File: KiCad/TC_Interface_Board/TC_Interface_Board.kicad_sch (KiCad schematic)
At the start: 23 parts, among them J1_24V_ROW1 Conn_01x04, J1_CN1_24V1 Conn_01x03, J2_CN2_9V_Main1 Conn_01x02, J3_CN3_9V_Main1 Conn_01x02, J4_BUS_MONITER1 Conn_01x05, Q1 DTC143E, Q2 DTC143E, U1 MC34063AP

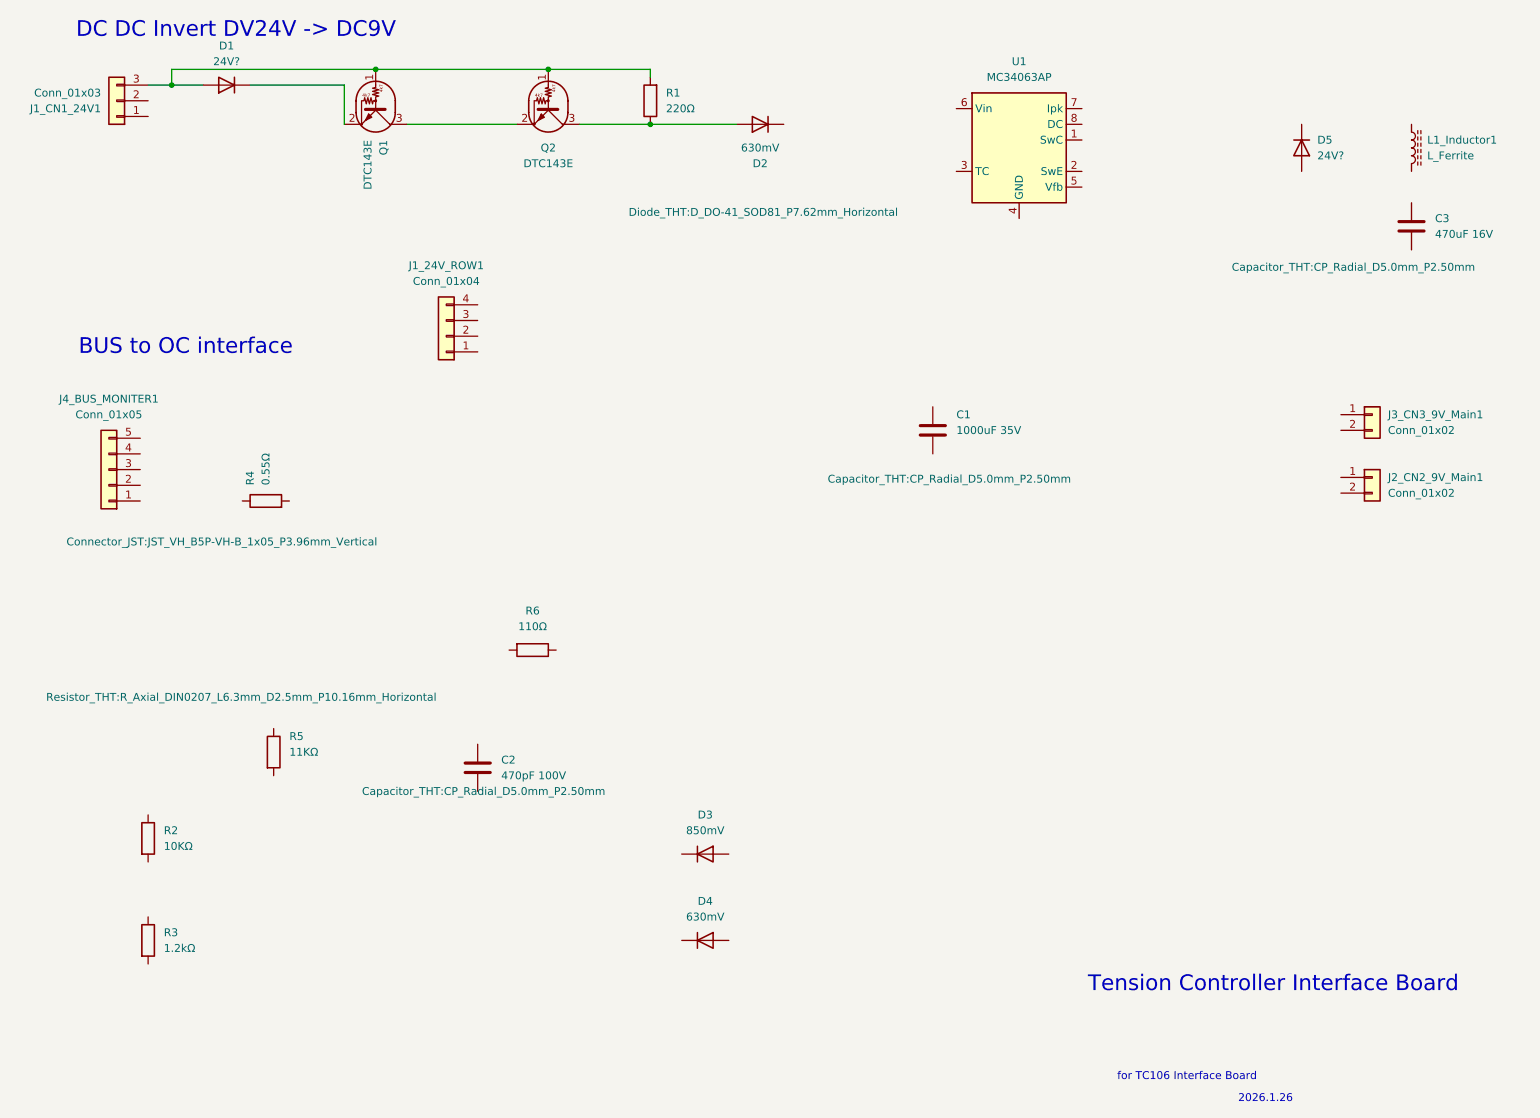
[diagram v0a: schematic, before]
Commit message: UPDATE
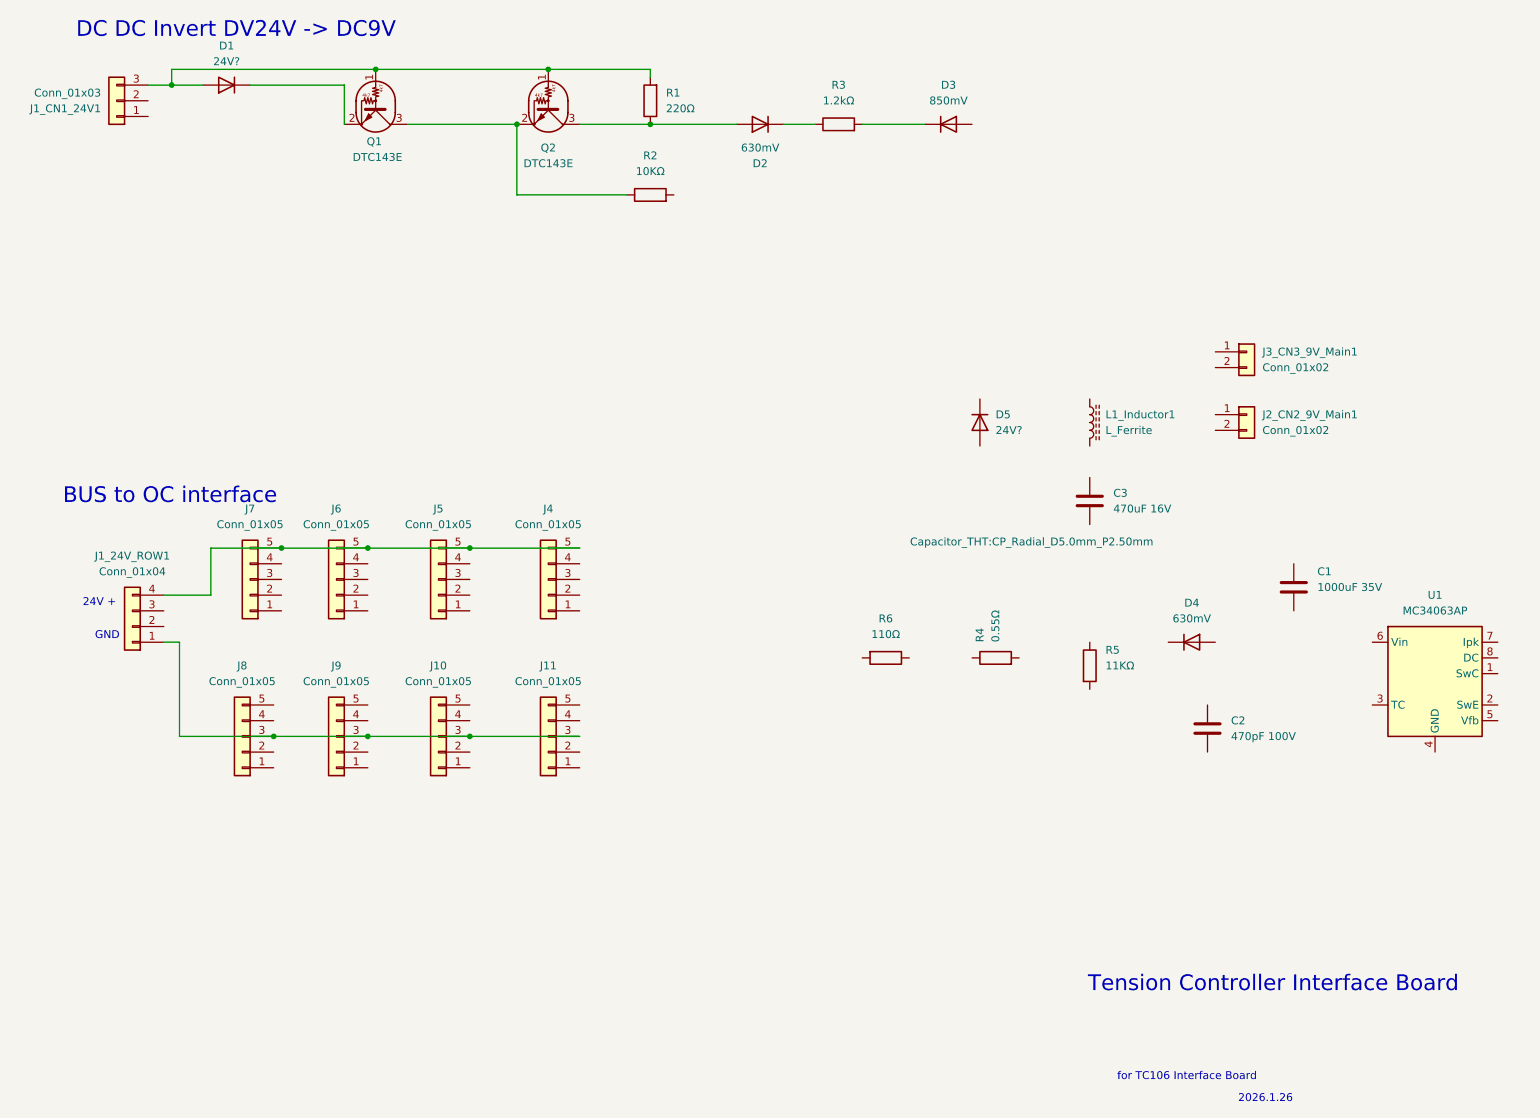
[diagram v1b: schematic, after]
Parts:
- added J10, J11, J5, J6, J7, J8, J9: Conn_01x05, Connector_JST:JST_VH_B5P-VH-B_1x05_P3.96mm_Vertical, symbol Connector_Generic:Conn_01x05
- D3: footprint Diode_THT:D_DO-41_SOD81_P7.62mm_Horizontal -> Diode_THT:D_DO-41_SOD81_P10.16mm_Horizontal
- R3: footprint Resistor_THT:R_Axial_DIN0207_L6.3mm_D2.5mm_P7.62mm_Horizontal -> Resistor_THT:R_Axial_DIN0207_L6.3mm_D2.5mm_P15.24mm_Horizontal
- renumbered J4_BUS_MONITER1 to J4
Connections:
- net at R3.1: now also D2.1 (K)
- net at R3.2: now also D3.1 (K)
- net at Q1.3 (C), Q2.2 (E): now also R2.1
- net at J1_24V_ROW1.1 (Pin_1): now also J10.3 (Pin_3), J11.3 (Pin_3), J8.3 (Pin_3), J9.3 (Pin_3)
- net at J1_24V_ROW1.4 (Pin_4): now also J4.5 (Pin_5), J5.5 (Pin_5), J6.5 (Pin_5), J7.5 (Pin_5)
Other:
- note added: "24V +"
- note added: "GND"
- moved on the sheet: C1, C2, C3, D3, D4, D5, J1_24V_ROW1, J2_CN2_9V_Main1, J3_CN3_9V_Main1, J4, L1_Inductor1, R2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

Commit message: UPDATE
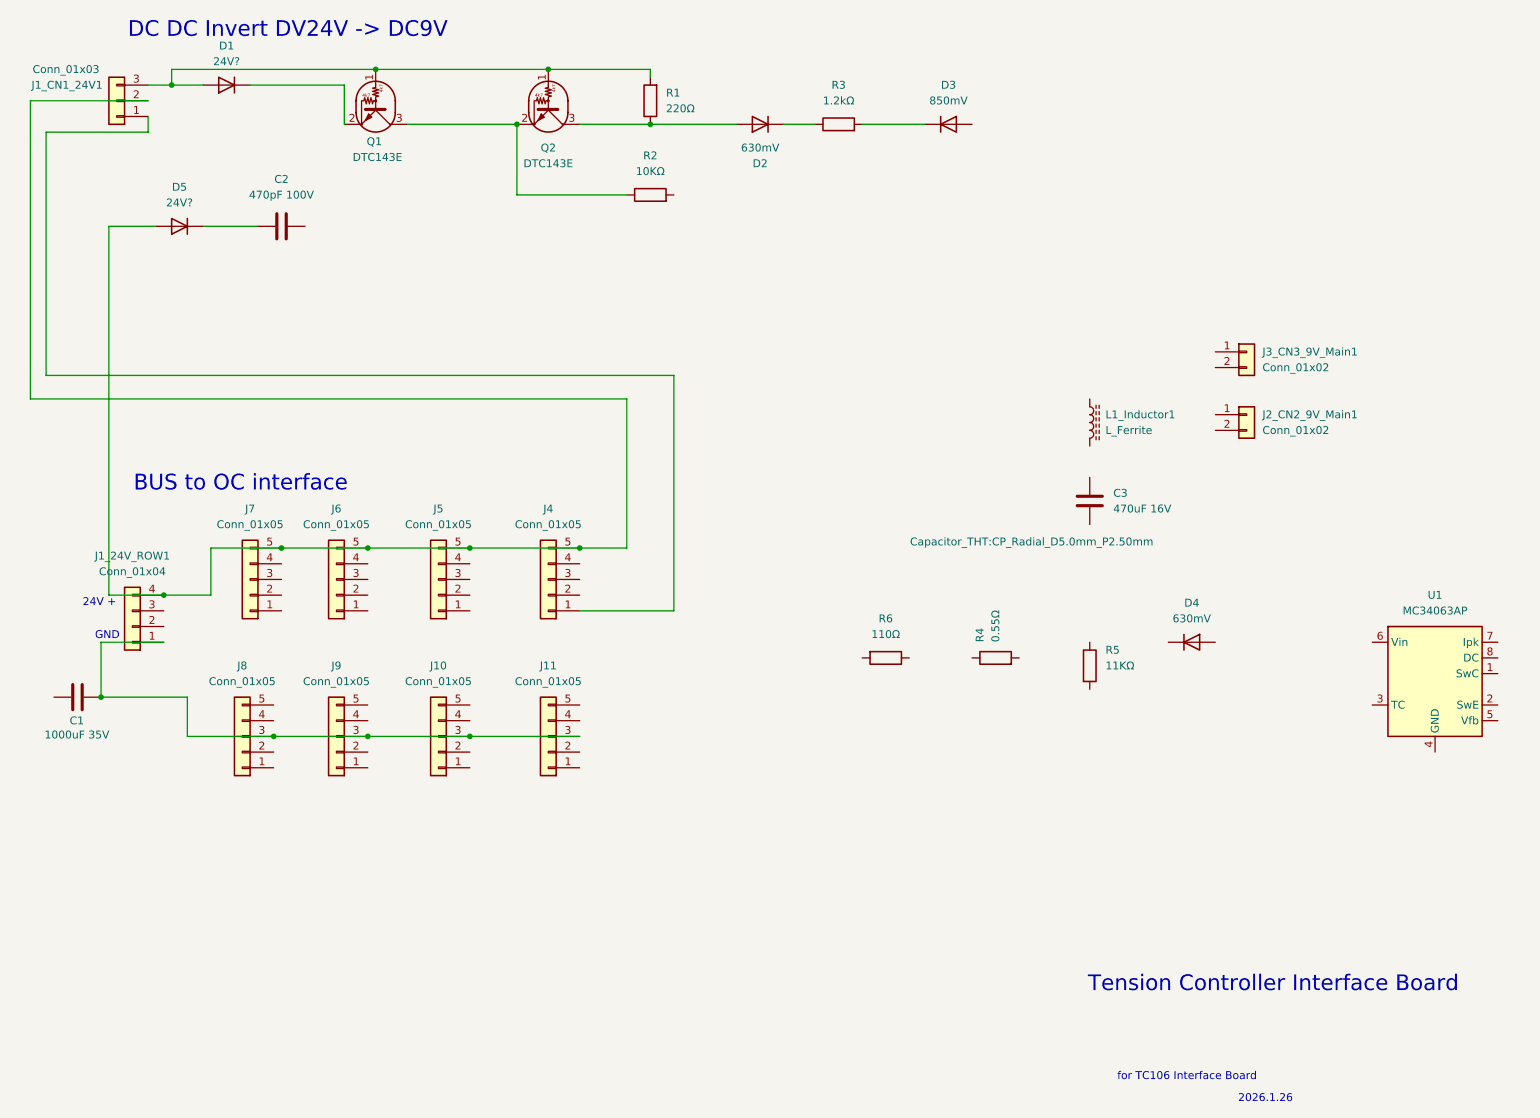
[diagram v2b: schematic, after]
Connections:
- net at D5.1 (K): now also C2.1
- net at D5.2 (A): now also J1_24V_ROW1.4 (Pin_4), J1_CN1_24V1.2 (Pin_2), J4.5 (Pin_5), J5.5 (Pin_5), J6.5 (Pin_5), J7.5 (Pin_5)
- net at J10.3 (Pin_3), J11.3 (Pin_3), J1_24V_ROW1.1 (Pin_1)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: now also C1.2
- net at J1_CN1_24V1.1 (Pin_1): now also J4.1 (Pin_1)
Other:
- moved on the sheet: C1, C2, D5
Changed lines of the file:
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@@
 	(text "BUS to OC interface"
 		(exclude_from_sim no)
-		(at 36.576 95.758 0)
+		(at 48.006 93.726 0)
 		(effects
 			(font
@@
 	(text "DC DC Invert DV24V -> DC9V"
 		(exclude_from_sim no)
-		(at 47.244 20.32 0)
+		(at 55.626 20.32 0)
 		(effects
 			(font
@@
 	)
 	(junction
+		(at 25.4 128.27)
+		(diameter 0)
+		(color 0 0 0 0)
+	)
+	(junction
 		(at 97.79 26.67)
 		(diameter 0)
@@
 	)
 	(junction
-		(at 53.34 134.62)
-		(diameter 0)
-		(color 0 0 0 0)
-	)
-	(junction
 		(at 69.85 26.67)
 		(diameter 0)
@@
 	)
 	(junction
+		(at 102.87 104.14)
+		(diameter 0)
+		(color 0 0 0 0)
+	)
+	(junction
+		(at 35.56 111.76)
+		(diameter 0)
+		(color 0 0 0 0)
+	)
+	(junction
 		(at 114.3 35.56)
+		(diameter 0)
+		(color 0 0 0 0)
+	)
+	(junction
+		(at 53.34 134.62)
 		(diameter 0)
 		(color 0 0 0 0)
@@
 	(wire
 		(pts
+			(xy 26.67 52.07) (xy 34.29 52.07)
+		)
+		(stroke
+			(width 0)
+			(type default)
+		)
+	)
+	(wire
+		(pts
 			(xy 33.02 29.21) (xy 36.83 29.21)
 		)
@@
 	(wire
 		(pts
+			(xy 35.56 111.76) (xy 26.67 111.76)
+		)
+		(stroke
+			(width 0)
+			(type default)
+		)
+	)
+	(wire
+		(pts
 			(xy 54.61 104.14) (xy 68.58 104.14)
 		)
@@
 	(wire
 		(pts
+			(xy 118.11 76.2) (xy 16.51 76.2)
+		)
+		(stroke
+			(width 0)
+			(type default)
+		)
+	)
+	(wire
+		(pts
 			(xy 74.93 35.56) (xy 92.71 35.56)
 		)
@@
 	(wire
 		(pts
+			(xy 39.37 128.27) (xy 25.4 128.27)
+		)
+		(stroke
+			(width 0)
+			(type default)
+		)
+	)
+	(wire
+		(pts
 			(xy 114.3 26.67) (xy 97.79 26.67)
 		)
@@
 	(wire
 		(pts
+			(xy 41.91 52.07) (xy 50.8 52.07)
+		)
+		(stroke
+			(width 0)
+			(type default)
+		)
+	)
+	(wire
+		(pts
+			(xy 33.02 36.83) (xy 33.02 34.29)
+		)
+		(stroke
+			(width 0)
+			(type default)
+		)
+	)
+	(wire
+		(pts
 			(xy 49.53 29.21) (xy 64.77 29.21)
 		)
@@
 	(wire
 		(pts
+			(xy 26.67 111.76) (xy 26.67 52.07)
+		)
+		(stroke
+			(width 0)
+			(type default)
+		)
+	)
+	(wire
+		(pts
+			(xy 25.4 119.38) (xy 25.4 128.27)
+		)
+		(stroke
+			(width 0)
+			(type default)
+		)
+	)
+	(wire
+		(pts
 			(xy 114.3 35.56) (xy 128.27 35.56)
 		)
@@
 	(wire
 		(pts
+			(xy 33.02 31.75) (xy 13.97 31.75)
+		)
+		(stroke
+			(width 0)
+			(type default)
+		)
+	)
+	(wire
+		(pts
 			(xy 64.77 29.21) (xy 64.77 35.56)
 		)
@@
 	(wire
 		(pts
+			(xy 110.49 80.01) (xy 110.49 104.14)
+		)
+		(stroke
+			(width 0)
+			(type default)
+		)
+	)
+	(wire
+		(pts
 			(xy 43.18 104.14) (xy 54.61 104.14)
 		)
@@
 	(wire
 		(pts
+			(xy 102.87 114.3) (xy 118.11 114.3)
+		)
+		(stroke
+			(width 0)
+			(type default)
+		)
+	)
+	(wire
+		(pts
 			(xy 148.59 35.56) (xy 158.75 35.56)
 		)
@@
 	(wire
 		(pts
+			(xy 53.34 134.62) (xy 39.37 134.62)
+		)
+		(stroke
+			(width 0)
+			(type default)
+		)
+	)
+	(wire
+		(pts
 			(xy 35.56 111.76) (xy 43.18 111.76)
 		)
@@
 	(wire
 		(pts
-			(xy 38.1 134.62) (xy 53.34 134.62)
-		)
-		(stroke
-			(width 0)
-			(type default)
-		)
-	)
-	(wire
-		(pts
-			(xy 35.56 119.38) (xy 38.1 119.38)
+			(xy 39.37 134.62) (xy 39.37 128.27)
+		)
+		(stroke
+			(width 0)
+			(type default)
+		)
+	)
+	(wire
+		(pts
+			(xy 13.97 31.75) (xy 13.97 80.01)
+		)
+		(stroke
+			(width 0)
+			(type default)
+		)
+	)
+	(wire
+		(pts
+			(xy 13.97 80.01) (xy 110.49 80.01)
+		)
+		(stroke
+			(width 0)
+			(type default)
+		)
+	)
+	(wire
+		(pts
+			(xy 16.51 36.83) (xy 33.02 36.83)
 		)
 		(stroke
@@
 	(wire
 		(pts
+			(xy 118.11 114.3) (xy 118.11 76.2)
+		)
+		(stroke
+			(width 0)
+			(type default)
+		)
+	)
+	(wire
+		(pts
+			(xy 35.56 119.38) (xy 25.4 119.38)
+		)
+		(stroke
+			(width 0)
+			(type default)
+		)
+	)
+	(wire
+		(pts
 			(xy 36.83 26.67) (xy 36.83 29.21)
 		)
@@
 	(wire
 		(pts
-			(xy 38.1 119.38) (xy 38.1 134.62)
+			(xy 16.51 76.2) (xy 16.51 36.83)
+		)
+		(stroke
+			(width 0)
+			(type default)
+		)
+	)
+	(wire
+		(pts
+			(xy 110.49 104.14) (xy 102.87 104.14)
 		)
 		(stroke
@@
 	(symbol
 		(lib_id "Device:D")
-		(at 167.64 83.82 270)
+		(at 38.1 52.07 180)
 		(unit 1)
 		(exclude_from_sim no)
@@
 		(fields_autoplaced yes)
 		(property "Reference" "D5"
-			(at 170.18 82.5499 90)
-			(effects
-				(font
-					(size 1.27 1.27)
-				)
-				(justify left)
+			(at 38.1 45.72 0)
+			(effects
+				(font
+					(size 1.27 1.27)
+				)
 			)
 		)
 		(property "Value" "24V?"
-			(at 170.18 85.0899 90)
-			(effects
-				(font
-					(size 1.27 1.27)
-				)
-				(justify left)
+			(at 38.1 48.26 0)
+			(effects
+				(font
+					(size 1.27 1.27)
+				)
 			)
 		)
 		(property "Footprint" "Diode_THT:D_DO-41_SOD81_P7.62mm_Horizontal"
-			(at 167.64 83.82 0)
+			(at 38.1 52.07 0)
 			(effects
 				(font
@@
 		)
 		(property "Datasheet" "~"
-			(at 167.64 83.82 0)
+			(at 38.1 52.07 0)
 			(effects
 				(font
@@
 		)
 		(property "Description" "Diode"
-			(at 167.64 83.82 0)
+			(at 38.1 52.07 0)
 			(effects
 				(font
@@
 		)
 		(property "Sim.Device" "D"
-			(at 167.64 83.82 0)
+			(at 38.1 52.07 0)
 			(effects
 				(font
@@
 		)
 		(property "Sim.Pins" "1=K 2=A"
-			(at 167.64 83.82 0)
+			(at 38.1 52.07 0)
 			(effects
 				(font
@@
 	(symbol
 		(lib_id "Device:C")
-		(at 218.44 110.49 180)
+		(at 21.59 128.27 90)
 		(unit 1)
 		(exclude_from_sim no)
@@
 		(dnp no)
 		(property "Reference" "C1"
-			(at 222.25 107.9499 0)
+			(at 20.32 132.08 90)
 			(effects
 				(font
@@
 		)
 		(property "Value" "1000uF 35V"
-			(at 222.25 110.4899 0)
+			(at 16.256 134.366 90)
 			(effects
 				(font
@@
 		)
 		(property "Footprint" "Capacitor_THT:CP_Radial_D5.0mm_P2.50mm"
-			(at 201.422 118.364 0)
+			(at 13.716 111.252 0)
 			(effects
 				(font
@@
 		)
 		(property "Datasheet" "~"
-			(at 218.44 110.49 0)
+			(at 21.59 128.27 0)
 			(effects
 				(font
@@
 		)
 		(property "Description" "Unpolarized capacitor"
-			(at 218.44 110.49 0)
+			(at 21.59 128.27 0)
 			(effects
 				(font
@@
 		(dnp no)
 		(property "Reference" "J1_CN1_24V1"
-			(at 25.4 33.0201 0)
+			(at 25.654 29.21 0)
 			(effects
 				(font
@@
 		)
 		(property "Value" "Conn_01x03"
-			(at 25.4 30.4801 0)
+			(at 25.146 26.67 0)
 			(effects
 				(font
@@
 	(symbol
 		(lib_id "Device:C")
-		(at 204.47 133.35 0)
+		(at 54.61 52.07 90)
 		(unit 1)
 		(exclude_from_sim no)
@@
 		(fields_autoplaced yes)
 		(property "Reference" "C2"
-			(at 208.28 132.0799 0)
-			(effects
-				(font
-					(size 1.27 1.27)
-				)
-				(justify left)
+			(at 54.61 44.45 90)
+			(effects
+				(font
+					(size 1.27 1.27)
+				)
 			)
 		)
 		(property "Value" "470pF 100V"
-			(at 208.28 134.6199 0)
-			(effects
-				(font
-					(size 1.27 1.27)
-				)
-				(justify left)
+			(at 54.61 46.99 90)
+			(effects
+				(font
+					(size 1.27 1.27)
+				)
 			)
 		)
 		(property "Footprint" "Capacitor_THT:CP_Radial_D5.0mm_P2.50mm"
-			(at 205.4352 137.16 0)
+			(at 58.42 51.1048 0)
 			(effects
 				(font
@@
 		)
 		(property "Datasheet" "~"
-			(at 204.47 133.35 0)
+			(at 54.61 52.07 0)
 			(effects
 				(font
@@
 		)
 		(property "Description" "Unpolarized capacitor"
-			(at 204.47 133.35 0)
-			(effects
-				(font
+			(at 54.61 52.07 0)
+			(effects
+				(font
